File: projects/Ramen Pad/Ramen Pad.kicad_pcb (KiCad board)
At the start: 2 copper layers, 85.7 x 123.8 mm, 75 parts, among them J1 USB4105-GF-A, K1 KEYSW, K10 KEYSW, K11 KEYSW, K12 KEYSW, K13 KEYSW, K14 KEYSW, K15 KEYSW, K16 KEYSW, K17 KEYSW, K2 KEYSW, K3 KEYSW, K4 KEYSW, K5 KEYSW, K6 KEYSW, K7 KEYSW, K8 KEYSW, K9 KEYSW, P1 CONN_3X2, SW1 Reset, U1 ATMEGA32U4, Y1 FA-238_16.0000MB-C3

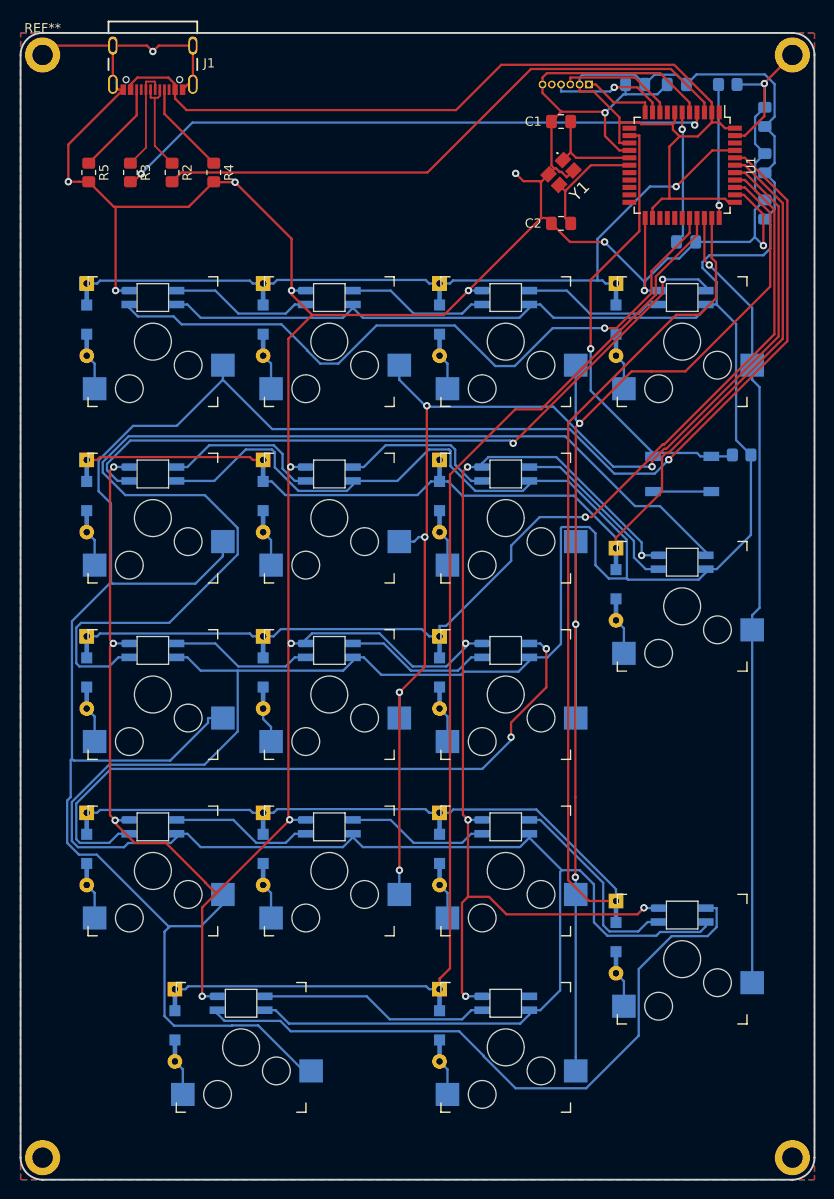
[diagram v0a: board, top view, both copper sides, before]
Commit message: PCB Update
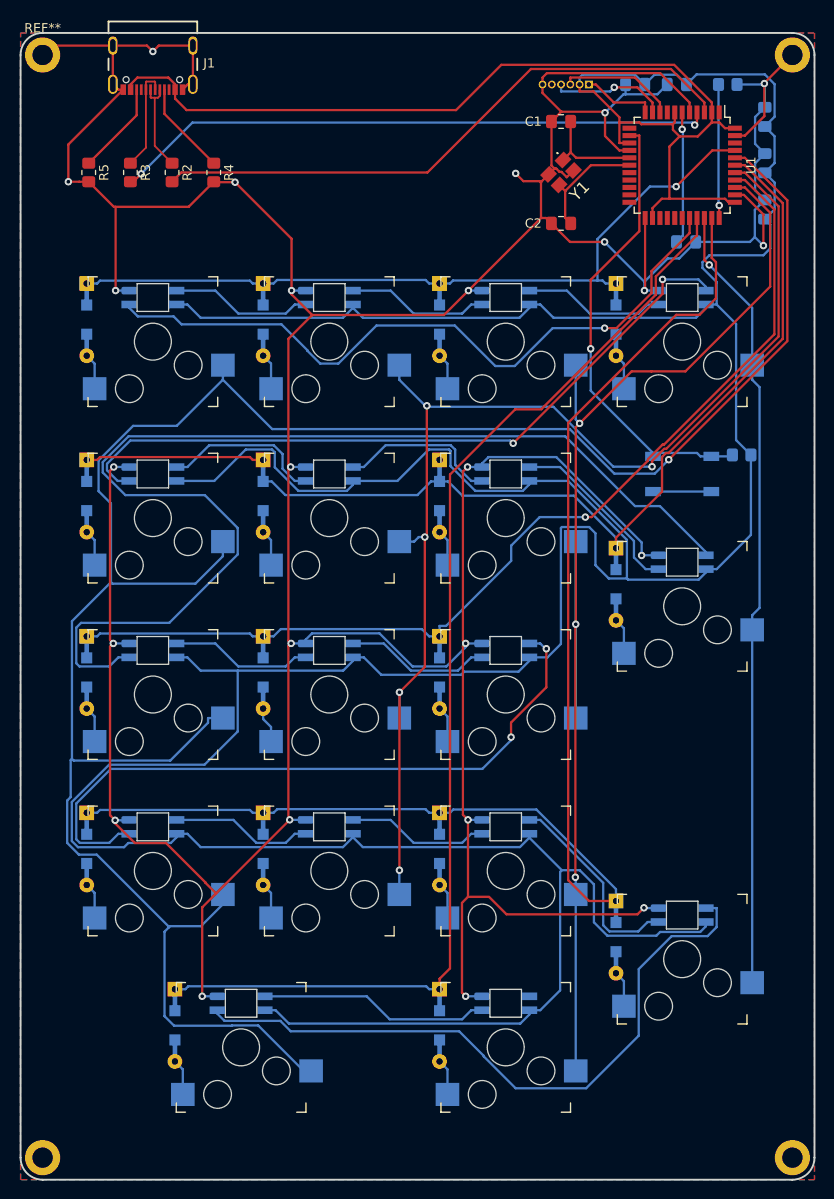
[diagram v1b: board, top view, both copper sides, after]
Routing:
- net /row0: track 90.8 -> 84.3 mm
- net /row3: track 157.9 -> 153.4 mm
- net /row1: track 123.3 -> 118.8 mm
- net /row2: track 116.4 -> 112.5 mm
- net /col0: track 241.1 -> 238.8 mm
- net /row4: track 129.9 -> 127.7 mm
- net GND: track 539.0 -> 537.3 mm
- net Net-(D9-Pad2): track 6.24 -> 5.11 mm
- net Net-(D8-Pad2): track 6.24 -> 5.11 mm
- net Net-(D7-Pad2): track 6.24 -> 5.11 mm
- net Net-(D6-Pad2): track 6.24 -> 5.11 mm
- net Net-(D5-Pad2): track 6.24 -> 5.11 mm
- net Net-(D4-Pad2): track 5.72 -> 4.60 mm
- net Net-(D3-Pad2): track 6.24 -> 5.11 mm
- net Net-(D2-Pad2): track 6.24 -> 5.11 mm
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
